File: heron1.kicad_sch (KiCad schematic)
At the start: 38 parts, among them J1 7.4 V BAT, J2 Conn_02x11_Counter_Clockwise, J3 MotorA, J4 Motor B, SW1 SW_Wuerth_450301014042, U1 ESP32-S3-DevKitC, U2 L7805, U4 L7806, U6 VNH5019A-E, U7 VNH5019A-E

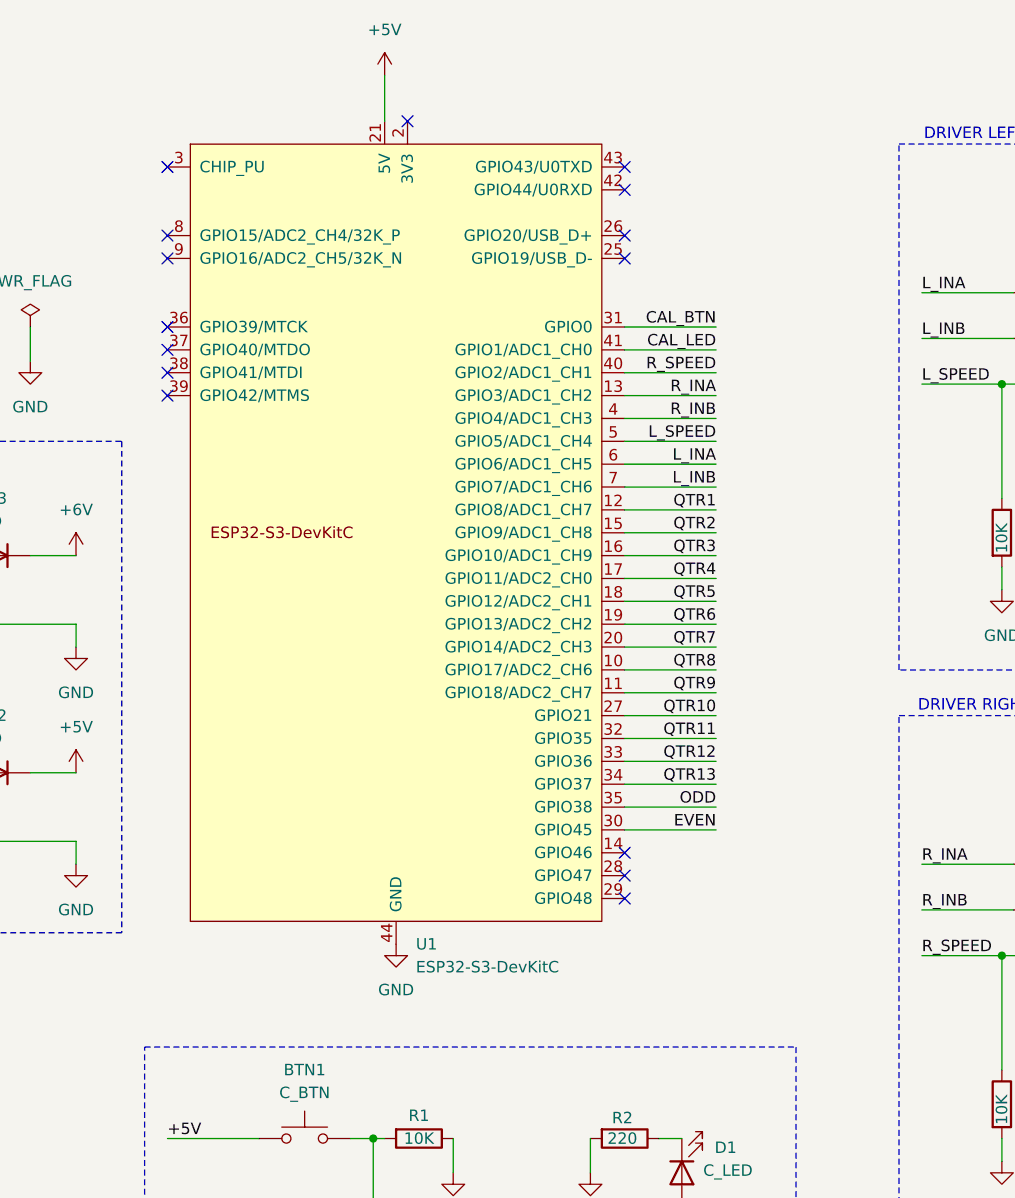
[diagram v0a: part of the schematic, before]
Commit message: first stage pcb
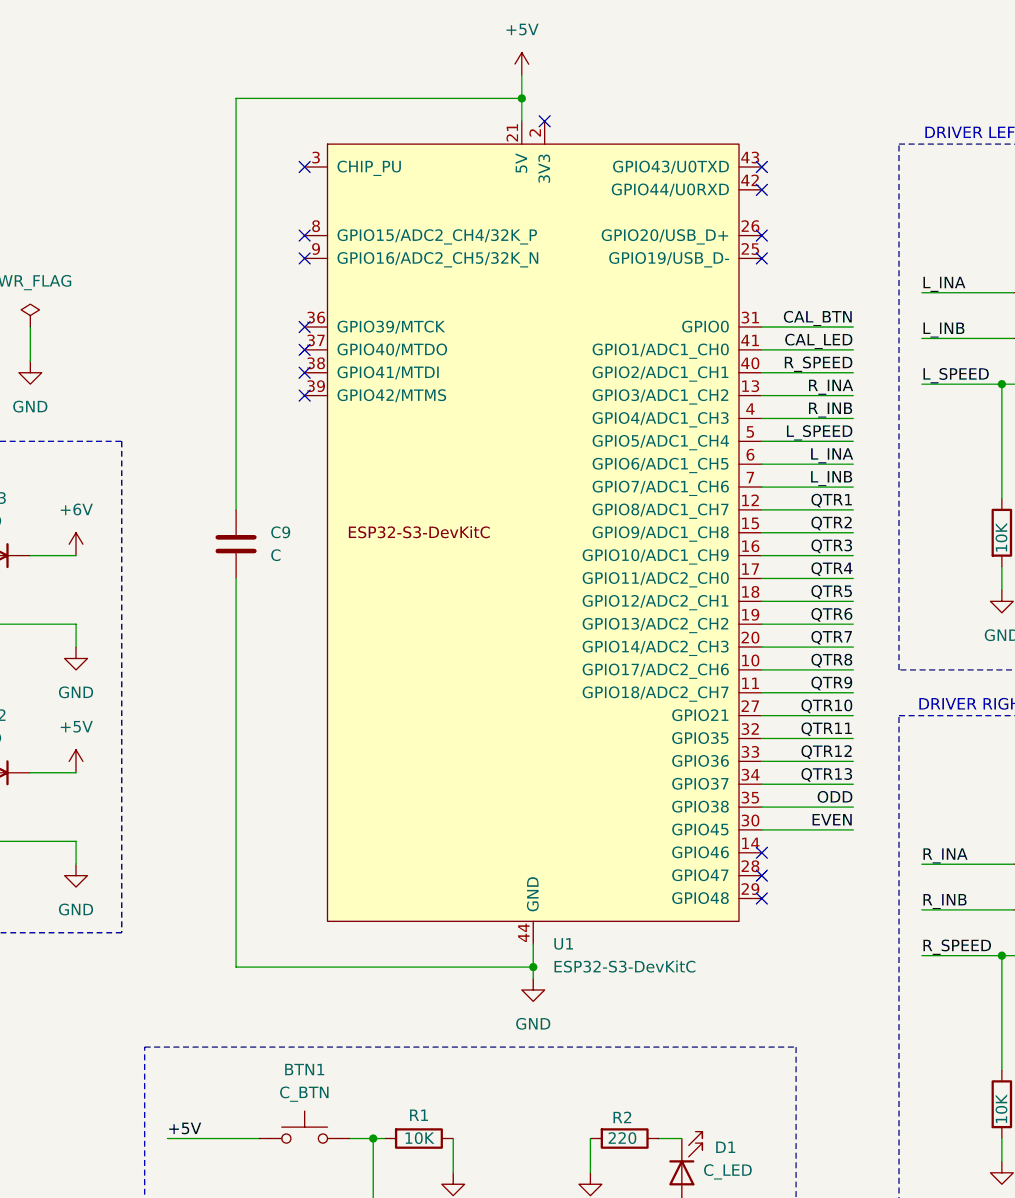
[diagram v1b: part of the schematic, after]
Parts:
- added C9: C, Capacitor_SMD:C_0805_2012Metric, symbol Device:C
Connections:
- net +5V: now also C9.1
- net GND: now also C9.2
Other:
- moved on the sheet: U1
